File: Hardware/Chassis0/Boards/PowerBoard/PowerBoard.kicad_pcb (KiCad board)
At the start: 4 copper layers, 180 x 110 mm, 83 parts, among them IC1 ACS772ECB-400B-PFF-T, IC2 ACS772ECB-400B-PFF-T, IC3 ACS772ECB-400B-PFF-T, IC4 ACS772ECB-400B-PFF-T, J1 Conn_02x08_Counter_Clockwise, J2 7466205R, J3 7466205R, J4 7466205R, J5 Conn_02x08_Counter_Clockwise, J6 7466205R, J7 Conn_02x08_Counter_Clockwise, J8 7466205R, J9 Conn_02x08_Counter_Clockwise, Q1 IPB017N10N5ATMA1, Q10 IPB017N10N5ATMA1, Q11 IPB017N10N5ATMA1, Q12 IPB017N10N5ATMA1, Q2 IPB017N10N5ATMA1, Q3 IPB017N10N5ATMA1, Q4 IPB017N10N5ATMA1, Q5 IPB017N10N5ATMA1, Q6 IPB017N10N5ATMA1, Q7 IPB017N10N5ATMA1, Q8 IPB017N10N5ATMA1, Q9 IPB017N10N5ATMA1, U1 LMT87DCK

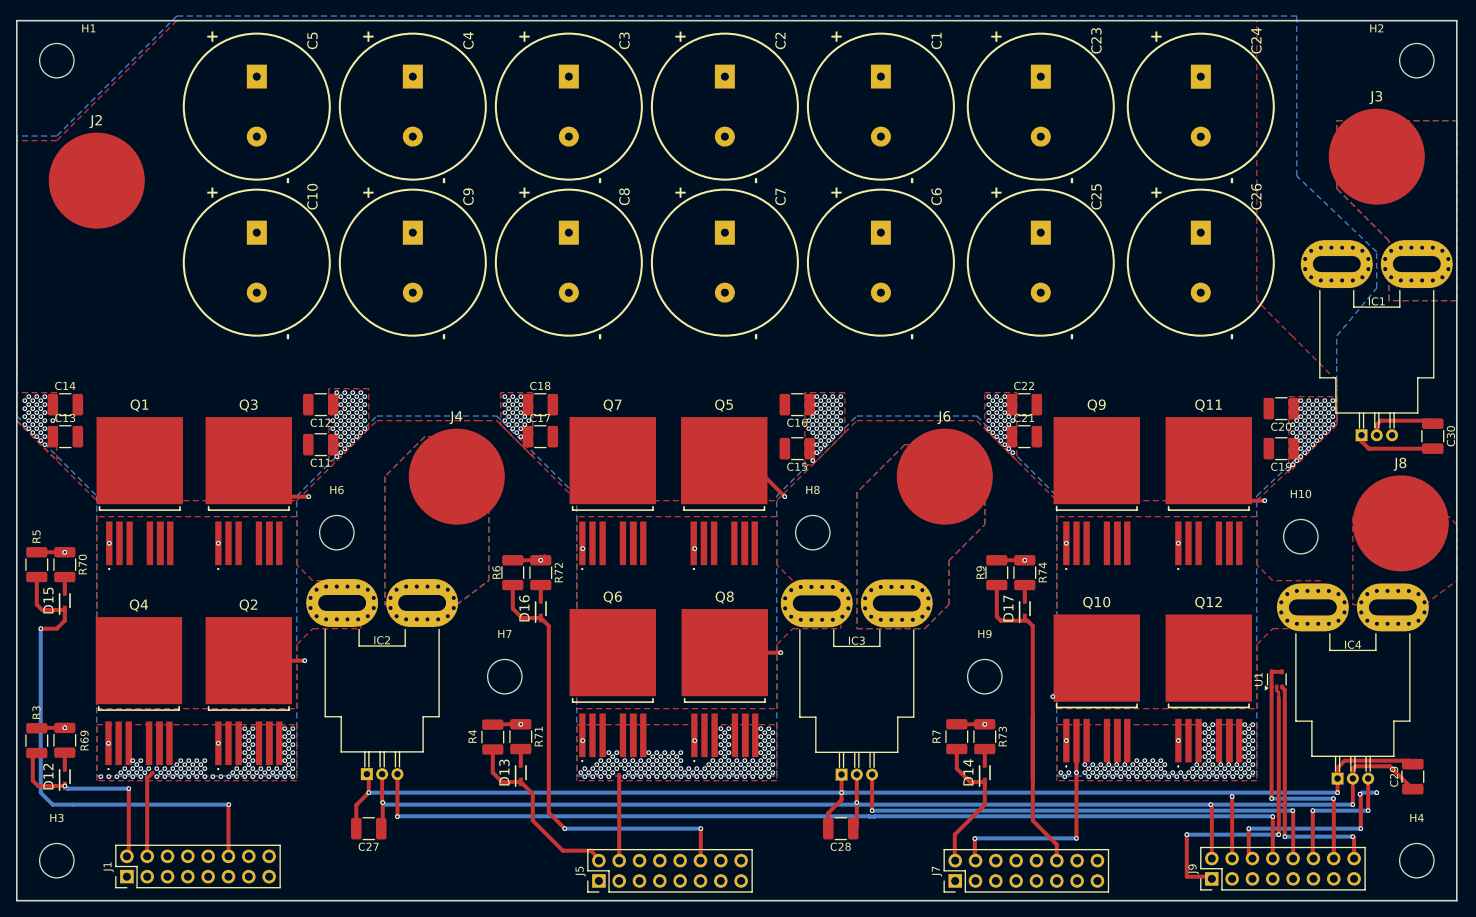
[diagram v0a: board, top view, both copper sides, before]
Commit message: finish chassis 0 board design v1
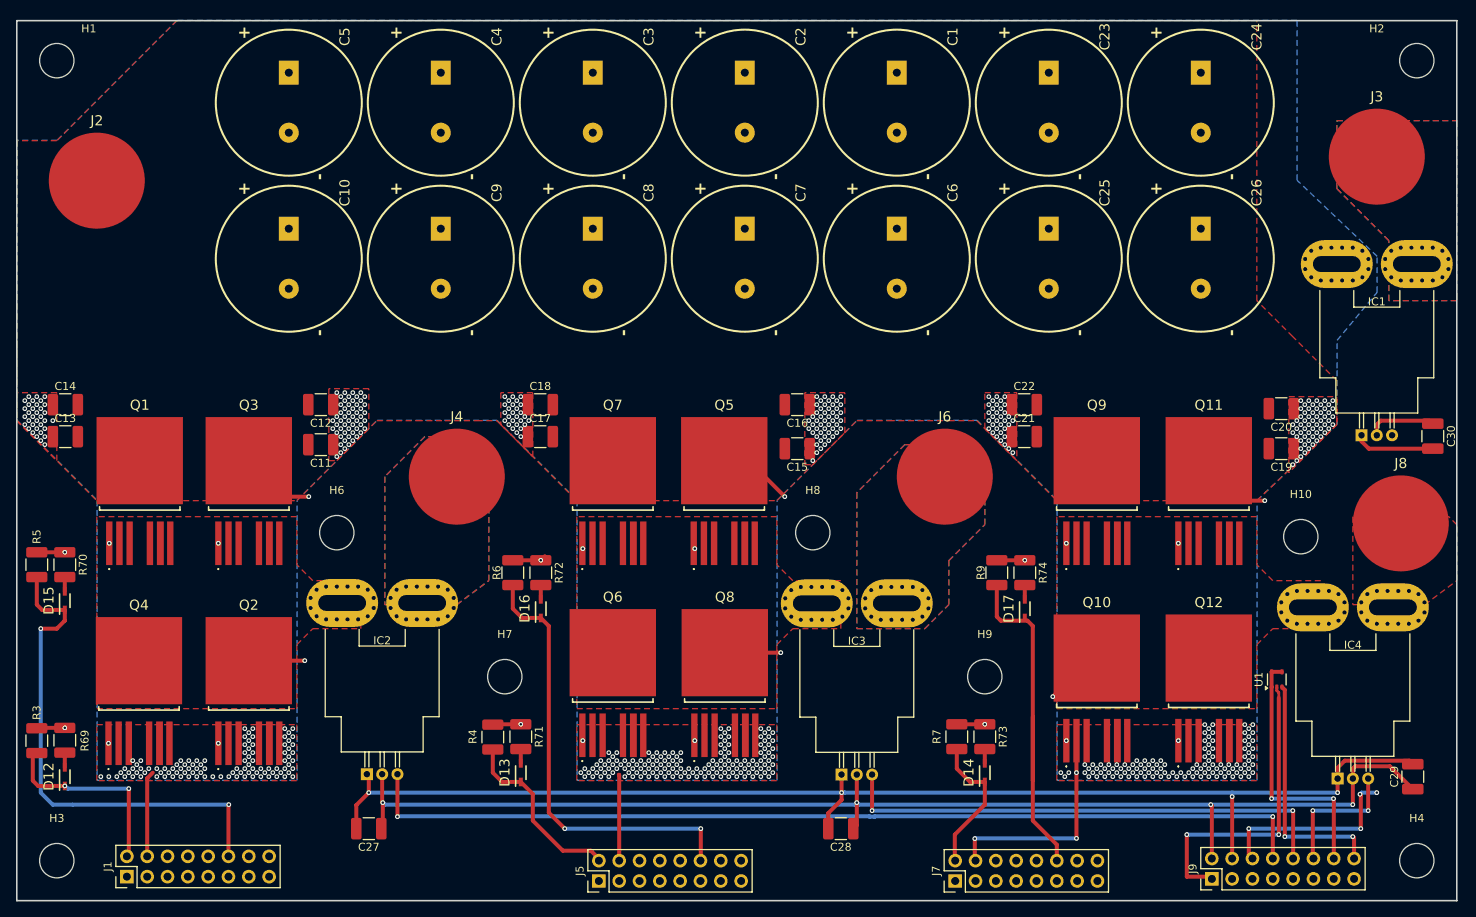
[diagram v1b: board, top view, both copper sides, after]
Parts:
- moved C10 4.03 mm to (34.0, 26.0)
- moved C5 4.03 mm to (34.0, 6.50)
- moved C4 3.53 mm to (53.0, 6.50)
- moved C9 3.53 mm to (53.0, 26.0)
- moved C3 3.03 mm to (72.0, 6.50)
- moved C8 3.03 mm to (72.0, 26.0)
- moved C2 2.54 mm to (91.0, 6.50)
- moved C7 2.54 mm to (91.0, 26.0)
- moved C1 2.05 mm to (110.0, 6.50)
- moved C6 2.05 mm to (110.0, 26.0)
- moved C23 1.12 mm to (129.0, 6.50)
- moved C25 1.12 mm to (129.0, 26.0)
- moved C24 0.50 mm to (148.0, 6.50)
- moved C26 0.50 mm to (148.0, 26.0)
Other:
- board text added: "todo: add ground planes model+serial number variants and other info warning labels design authors (konstantin/thomas)"
- board text removed: "todo: move power to right side (both dc terminals are on right side) add ground planes maybe 2nd temp sense model+serial number variants and other info warning labels design authors (konstantin/thomas)"
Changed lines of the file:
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@@
 		(locked yes)
 		(layer "F.Cu")
-		(at 49.504 6.996 -90)
+		(at 53 6.504 -90)
 		(descr "18mm x 30.5mm")
 		(tags "Capacitor")
@@
 		(locked yes)
 		(layer "F.Cu")
-		(at 69.008 6.996 -90)
+		(at 72 6.504 -90)
 		(descr "18mm x 30.5mm")
 		(tags "Capacitor")
@@
 		(locked yes)
 		(layer "F.Cu")
-		(at 128 26.5 -90)
+		(at 129 26.004 -90)
 		(descr "18mm x 30.5mm")
 		(tags "Capacitor")
@@
 		(locked yes)
 		(layer "F.Cu")
-		(at 148 26.5 -90)
+		(at 148 26.004 -90)
 		(descr "18mm x 30.5mm")
 		(tags "Capacitor")
@@
 		(locked yes)
 		(layer "F.Cu")
-		(at 148 7 -90)
+		(at 148 6.504 -90)
 		(descr "18mm x 30.5mm")
 		(tags "Capacitor")
@@
 		(locked yes)
 		(layer "F.Cu")
-		(at 108.016 6.996 -90)
+		(at 110 6.5 -90)
 		(descr "18mm x 30.5mm")
 		(tags "Capacitor")
@@
 		(locked yes)
 		(layer "F.Cu")
-		(at 30 26.5 -90)
+		(at 34 26.008 -90)
 		(descr "18mm x 30.5mm")
 		(tags "Capacitor")
@@
 		(locked yes)
 		(layer "F.Cu")
-		(at 88.512 26.5 -90)
+		(at 91 26.004 -90)
 		(descr "18mm x 30.5mm")
 		(tags "Capacitor")
@@
 		(locked yes)
 		(layer "F.Cu")
-		(at 128 7 -90)
+		(at 129 6.504 -90)
 		(descr "18mm x 30.5mm")
 		(tags "Capacitor")
@@
 		(locked yes)
 		(layer "F.Cu")
-		(at 108.016 26.5 -90)
+		(at 110 26.004 -90)
 		(descr "18mm x 30.5mm")
 		(tags "Capacitor")
@@
 		(locked yes)
 		(layer "F.Cu")
-		(at 88.512 6.996 -90)
+		(at 91 6.5 -90)
 		(descr "18mm x 30.5mm")
 		(tags "Capacitor")
@@
 		(locked yes)
 		(layer "F.Cu")
-		(at 49.504 26.5 -90)
+		(at 53 26.008 -90)
 		(descr "18mm x 30.5mm")
 		(tags "Capacitor")
@@
 		(locked yes)
 		(layer "F.Cu")
-		(at 30 6.996 -90)
+		(at 34 6.504 -90)
 		(descr "18mm x 30.5mm")
 		(tags "Capacitor")
@@
 		(locked yes)
 		(layer "F.Cu")
-		(at 69.008 26.5 -90)
+		(at 72 26.008 -90)
 		(descr "18mm x 30.5mm")
 		(tags "Capacitor")
@@
 		(layer "Edge.Cuts")
 	)
-	(gr_text "todo:\nmove power to right side (both dc terminals are on right side)\nadd ground planes\nmaybe 2nd temp sense\nmodel+serial number\nvariants and other info\nwarning labels\ndesign authors (konstantin/thomas)"
+	(gr_text "todo:\nadd ground planes\nmodel+serial number\nvariants and other info\nwarning labels\ndesign authors (konstantin/thomas)"
 		(at 181 -2 0)
 		(layer "Edge.Cuts")
@@
 		(polygon
 			(pts
-				(xy 20 -0.581967) (xy 5 14.418033) (xy 0 14.418033) (xy 0 44.418033) (xy 0 49.418033) (xy 10 59.418033)
-				(xy 10 94.418033) (xy 35 94.418033) (xy 35 59.418033) (xy 45 49.418033) (xy 60 49.418033) (xy 70 59.418033)
-				(xy 70 94.418033) (xy 95 94.418033) (xy 95 59.418033) (xy 105 49.418033) (xy 120 49.418033) (xy 130 59.418033)
-				(xy 130 94.418033) (xy 155 94.418033) (xy 155 59.418033) (xy 165 49.918033) (xy 165 42.918033) (xy 165 39.418033)
-				(xy 170 33.418033) (xy 170 28.918033) (xy 160 19.418033) (xy 160 -0.581967)
+				(xy 20.040984 -0.040984) (xy 5.040984 14.959016) (xy 0.040984 14.959016) (xy 0.040984 44.959016)
+				(xy 0.040984 49.959016) (xy 10.040984 59.959016) (xy 10.040984 94.959016) (xy 35.040984 94.959016)
+				(xy 35.040984 59.959016) (xy 45.040984 49.959016) (xy 60.040984 49.959016) (xy 70.040984 59.959016)
+				(xy 70.040984 94.959016) (xy 95.040984 94.959016) (xy 95.040984 59.959016) (xy 105.040984 49.959016)
+				(xy 120.040984 49.959016) (xy 130.040984 59.959016) (xy 130.040984 94.959016) (xy 155.040984 94.959016)
+				(xy 155.040984 59.959016) (xy 165.040984 50.459016) (xy 165.040984 43.459016) (xy 165.040984 39.959016)
+				(xy 170.040984 33.959016) (xy 170.040984 29.459016) (xy 160.040984 19.959016) (xy 160.040984 -0.040984)
 			)
 		)
